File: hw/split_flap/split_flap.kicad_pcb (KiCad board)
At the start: 2 copper layers, 85.5 x 67.2 mm, 41 parts, among them J1 Conn_01x02, J10 Conn_01x05, J11 Conn_01x05, J12 Conn_01x05, J13 Conn_01x05, J14 Conn_01x05, J17 EXPANDER_PORT, J19 POWER, J2 Conn_01x02, J21 Conn_01x05, J22 Conn_01x05, J3 Conn_01x02, J4 Conn_01x02, J5 Conn_01x02, J6 Conn_01x02, J7 Conn_01x02, J8 Conn_01x02, J9 Conn_01x05, U1 74HCT125, U10 ULN2803A, U14 ULN2803A, U2 NodeMCU_1.0_(ESP-12E), U3 74HC595, U4 PCF8574, U5 74HC595, U6 ULN2803A, U7 74HC595, U8 ULN2803A, U9 74HC595

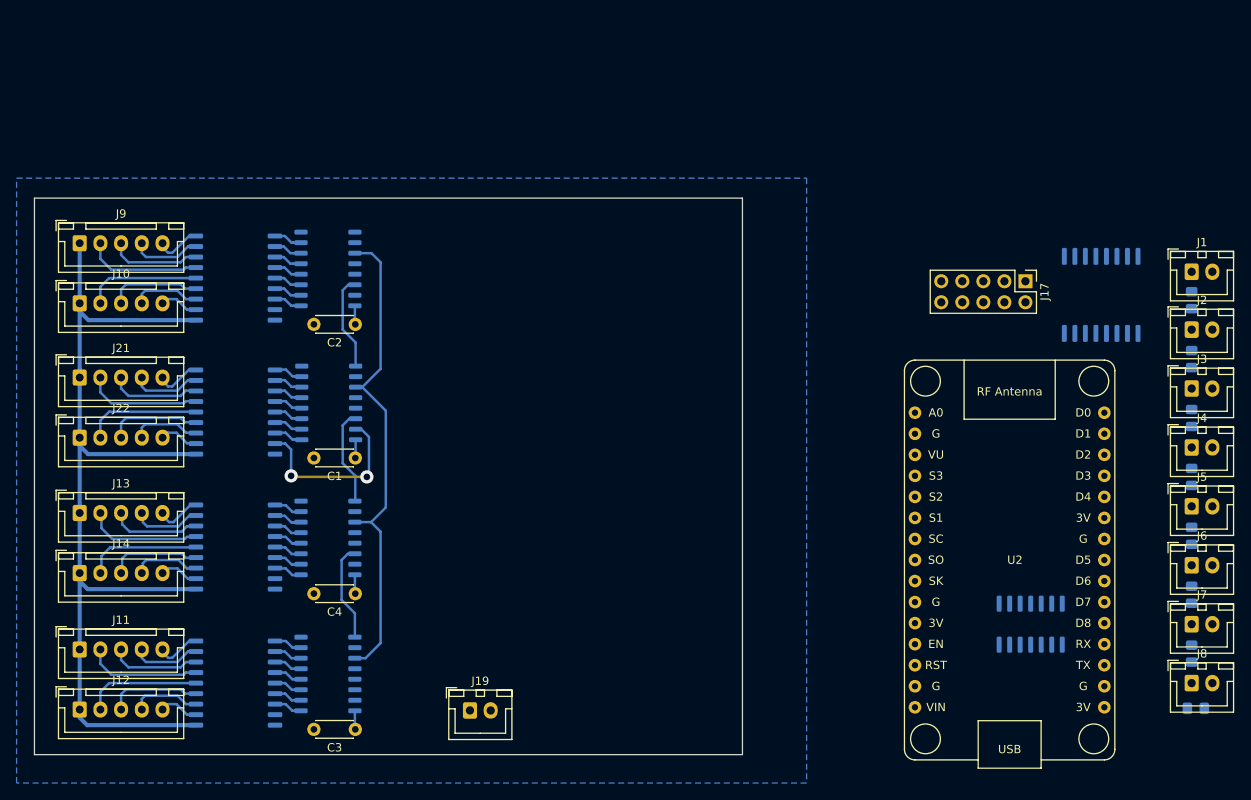
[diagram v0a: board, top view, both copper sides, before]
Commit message: Route new PCB completely.
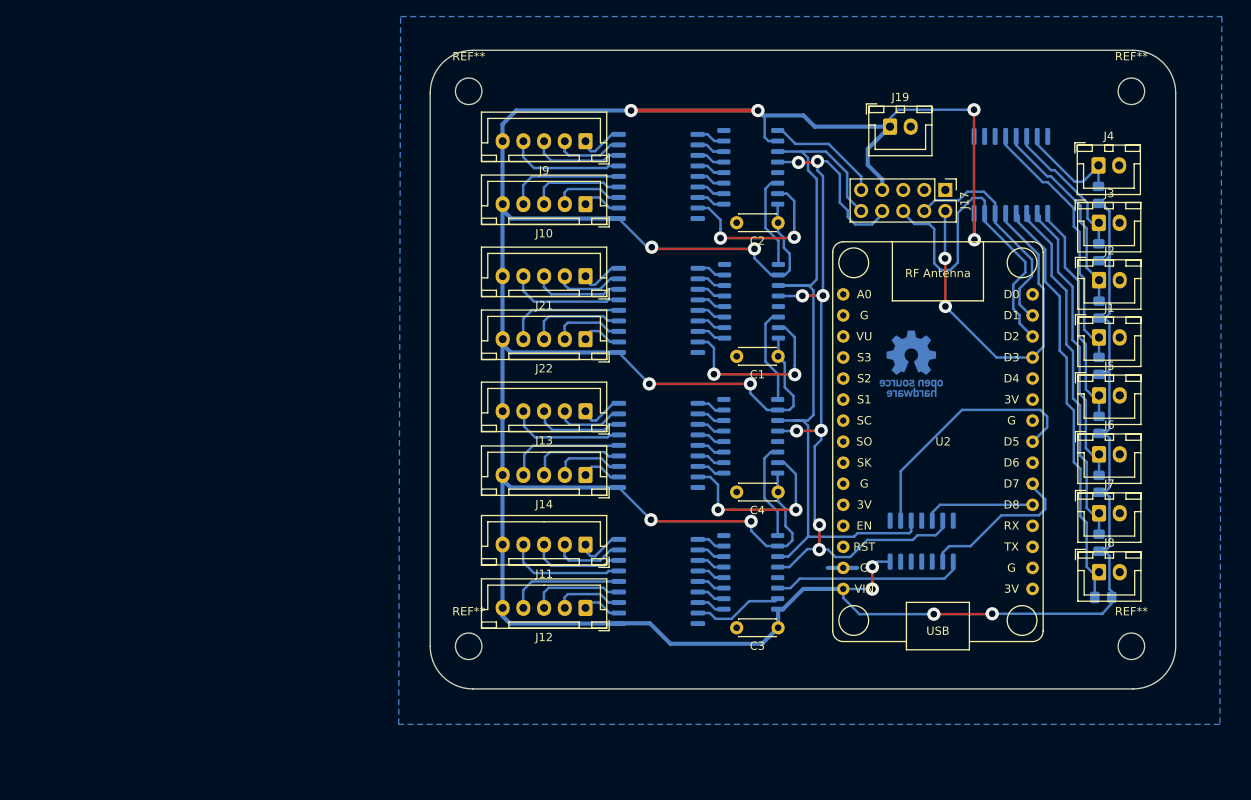
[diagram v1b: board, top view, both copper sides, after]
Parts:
- added REF**: OSHW-Logo_7.5x8mm_Copper, Symbol:OSHW-Logo_7.5x8mm_Copper, B.Cu at (153.5, 92.9)
- added REF**: MountingHole_3.2mm_M3, MountingHole:MountingHole_3.2mm_M3, F.Cu at (180.1, 127.0)
- added REF**: MountingHole_3.2mm_M3, MountingHole:MountingHole_3.2mm_M3, F.Cu at (100.0, 127.0)
- added REF**: MountingHole_3.2mm_M3, MountingHole:MountingHole_3.2mm_M3, F.Cu at (180.1, 60.0)
- added REF**: MountingHole_3.2mm_M3, MountingHole:MountingHole_3.2mm_M3, F.Cu at (100.0, 60.0)
- moved J19 86.8 mm to (150.9, 64.3)
- moved J11 62.4 mm to (114.2, 114.7), turned to 180 degrees
- moved J9 62.3 mm to (114.2, 66.0), turned to 180 degrees
- moved J13 62.3 mm to (114.2, 98.6), turned to 180 degrees
- moved J12 62.3 mm to (114.2, 122.4), turned to 180 degrees
- moved J21 62.3 mm to (114.2, 82.3), turned to 180 degrees
- moved J10 62.2 mm to (114.2, 73.6), turned to 180 degrees
- moved J22 62.2 mm to (114.2, 89.9), turned to 180 degrees
- moved J14 62.2 mm to (114.2, 106.3), turned to 180 degrees
- moved C1 52.5 mm to (137.4, 92.0)
- moved C2 52.5 mm to (137.4, 75.9)
- moved C3 52.5 mm to (137.4, 124.8)
- moved C4 52.5 mm to (137.4, 108.4)
- moved U10 52.5 mm to (122.9, 102.8)
- moved U14 52.5 mm to (122.9, 86.5)
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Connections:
- J10 pad 1: +5V -> /sheet5E0964A4/M7
- J10 pad 2: /sheet5E0964A4/M4 -> /sheet5E0964A4/M6
- J10 pad 4: /sheet5E0964A4/M6 -> /sheet5E0964A4/M4
- J10 pad 5: /sheet5E0964A4/M7 -> +5V
- J11 pad 1: +5V -> /sheet5E092C79/M0
- J11 pad 2: /sheet5E092C79/M3 -> /sheet5E092C79/M1
- J11 pad 4: /sheet5E092C79/M1 -> /sheet5E092C79/M3
- J11 pad 5: /sheet5E092C79/M0 -> +5V
- J12 pad 1: +5V -> /sheet5E092C79/M7
- J12 pad 2: /sheet5E092C79/M4 -> /sheet5E092C79/M6
- J12 pad 4: /sheet5E092C79/M6 -> /sheet5E092C79/M4
- J12 pad 5: /sheet5E092C79/M7 -> +5V
- J13 pad 1: +5V -> /sheet5E0B21A0/M0
- J13 pad 2: /sheet5E0B21A0/M3 -> /sheet5E0B21A0/M1
- J13 pad 4: /sheet5E0B21A0/M1 -> /sheet5E0B21A0/M3
- J13 pad 5: /sheet5E0B21A0/M0 -> +5V
- J14 pad 1: +5V -> /sheet5E0B21A0/M7
- J14 pad 2: /sheet5E0B21A0/M4 -> /sheet5E0B21A0/M6
- J14 pad 4: /sheet5E0B21A0/M6 -> /sheet5E0B21A0/M4
- J14 pad 5: /sheet5E0B21A0/M7 -> +5V
- J21 pad 1: +5V -> /sheet5DED9C19/M0
- J21 pad 2: /sheet5DED9C19/M3 -> /sheet5DED9C19/M1
- J21 pad 4: /sheet5DED9C19/M1 -> /sheet5DED9C19/M3
- J21 pad 5: /sheet5DED9C19/M0 -> +5V
- J22 pad 1: +5V -> /sheet5DED9C19/M7
- J22 pad 2: /sheet5DED9C19/M4 -> /sheet5DED9C19/M6
- J22 pad 4: /sheet5DED9C19/M6 -> /sheet5DED9C19/M4
- J22 pad 5: /sheet5DED9C19/M7 -> +5V
- J9 pad 1: +5V -> /sheet5E0964A4/M0
- J9 pad 2: /sheet5E0964A4/M3 -> /sheet5E0964A4/M1
- J9 pad 4: /sheet5E0964A4/M1 -> /sheet5E0964A4/M3
- J9 pad 5: /sheet5E0964A4/M0 -> +5V
- U2 pad 20: /SPI_3.3_DO -> /SPI_3.3_CS
- U2 pad 21: /SPI_3.3_CS -> /SPI_3.3_DO
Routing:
- net +5V: track 127.0 -> 445.7 mm, vias 0 -> 14
- net /SPI_CS: track 0.00 -> 101.3 mm, vias 0 -> 8
- net Net-(J8-Pad1): track 0.00 -> 51.2 mm
- net /INT: track 0.00 -> 44.5 mm, vias 0 -> 2
- net Net-(J7-Pad1): track 0.00 -> 42.8 mm
- net /SDA: track 0.00 -> 42.6 mm
- net Net-(J6-Pad1): track 0.00 -> 35.2 mm
- net /SPI_CLK: track 59.4 -> 93.6 mm
- net Net-(J1-Pad1): track 0.00 -> 31.2 mm
- net /SPI_3.3_CLK: track 0.00 -> 30.8 mm
- net /SCL: track 0.00 -> 26.9 mm
- net Net-(J5-Pad1): track 0.00 -> 26.7 mm
- net Net-(J2-Pad1): track 0.00 -> 24.3 mm
- net /SPI_DO: track 0.00 -> 23.1 mm
- net /sheet5E0B21A0/O1: track 0.00 -> 22.3 mm, vias 0 -> 2
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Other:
- board size 85.5 x 67.2 mm -> 90 x 77.1 mm
